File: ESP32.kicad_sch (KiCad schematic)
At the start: 5 parts, among them U1 ESP32-S3-MINI-1-N8

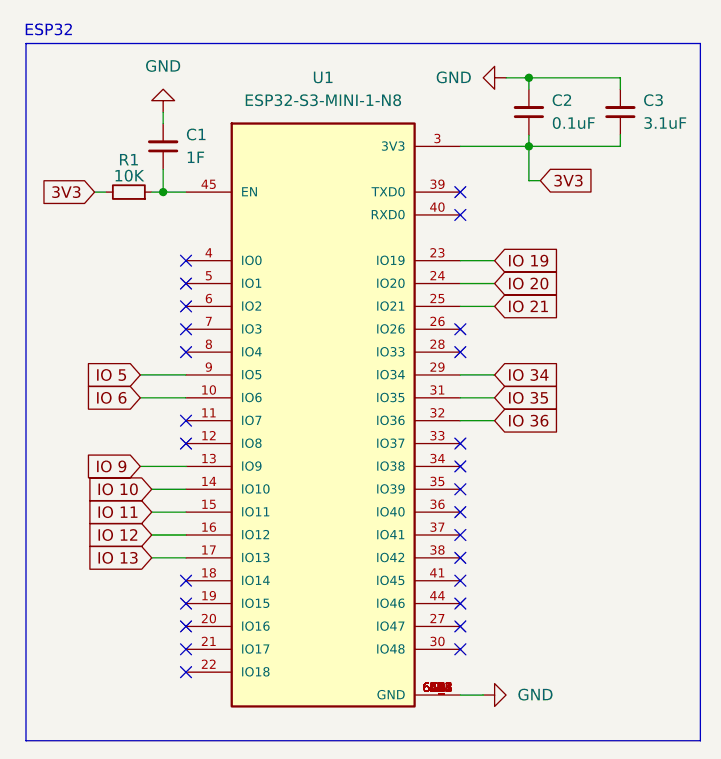
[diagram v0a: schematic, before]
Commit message: Create PCB
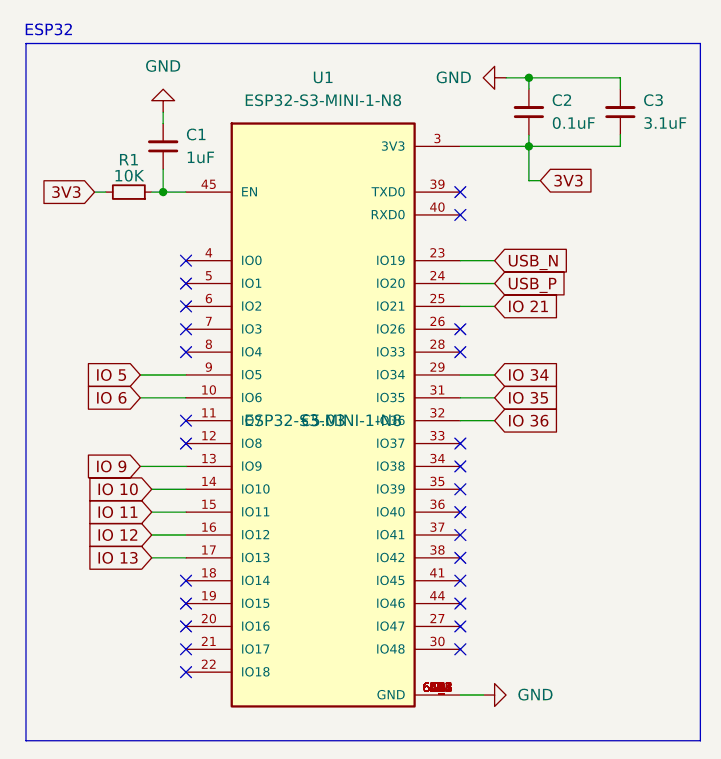
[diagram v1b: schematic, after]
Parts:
- C1: value 1F -> 1uF; DigiKey_Part_Number (none) -> 311-1445-1-ND; Manufacturer_Part_Number (none) -> CC0603KRX5R8BB105; Price (none) -> €0.95
- C2: DigiKey_Part_Number (none) -> 311-1341-1-ND; Manufacturer_Part_Number (none) -> CC0603KRX7R8BB104; Price (none) -> €0.48
- C3: footprint Capacitor_SMD:C_0603_1608Metric -> Capacitor_SMD:C_0805_2012Metric; DigiKey_Part_Number (none) -> 311-1190-1-ND; Manufacturer_Part_Number (none) -> CC0805ZKY5V6BB335; Price (none) -> €0.17
- R1: footprint Resistor_SMD:R_0603_1608Metric -> Resistor_SMD:R_0402_1005Metric; DigiKey_Part_Number (none) -> 311-10KJRCT-ND; Manufacturer_Part_Number (none) -> RC0402JR-0710KL; Price (none) -> €0.30
- U1: Check_prices https://www.snapeda.com/parts/ESP32-S3-MINI-1-N8/Espressif+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 -> (none); Description_1 Bluetooth, WiFi 802.11b/g/n, Bluetooth v5.0 Transceiver Mod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 -> (none); DigiKey_Part_Number 1965-ESP32-S3-MINI-1-N8TR-ND -> 1965-ESP32-S3-MINI-1-N8CT-ND; MANUFACTURER Espressif -> (none); MAXIMUM_PACKAGE_HEIGHT 2.55mm -> (none); MF Espressif Systems -> (none); MP ESP32-S3-MINI-1-N8 -> (none); Manufacturer_Part_Number (none) -> ESP32-S3-MINI-1-N8; PARTREV v0.6 -> (none); Package None -> (none); Price (none) -> €5.03; STANDARD Manufacturer Recommendations -> (none); SnapEDA_Link https://www.snapeda.com/parts/ESP32-S3-MINI-1-N8/Espressif+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 -> (none)
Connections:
- net IO 19 renamed USB_N
- net IO 20 renamed USB_P
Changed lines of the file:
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@@
 		)
 	)
-	(global_label "IO 19"
+	(global_label "USB_N"
 		(shape input)
 		(at 66.04 40.64 0)
@@
 		)
 		(property "Intersheetrefs" "${INTERSHEET_REFS}"
-			(at 74.3471 40.64 0)
+			(at 75.1333 40.64 0)
 			(effects
 				(font
@@
 		)
 	)
-	(global_label "IO 20"
+	(global_label "USB_P"
 		(shape input)
 		(at 66.04 43.18 0)
@@
 		)
 		(property "Intersheetrefs" "${INTERSHEET_REFS}"
-			(at 74.3471 43.18 0)
+			(at 75.0728 43.18 0)
 			(effects
 				(font
@@
 		(dnp no)
 		(fields_autoplaced yes)
-		(property "Reference" "#PWR042"
+		(property "Reference" "#PWR01"
 			(at 29.21 17.78 0)
 			(effects
@@
 			(project "RFID_Device"
 				(path "/f4733a35-9ae9-40ca-bc69-86dc96557334/b59a840b-0db4-4dd4-af14-dad68e1751ca"
-					(reference "#PWR042")
+					(reference "#PWR01")
 					(unit 1)
 				)
@@
 			)
 		)
-		(property "Value" "1F"
+		(property "Value" "1uF"
 			(at 31.75 29.2035 0)
 			(effects
@@
 		)
 		(property "Description" "Unpolarized capacitor, small symbol"
+			(at 29.21 27.94 0)
+			(effects
+				(font
+					(size 1.27 1.27)
+				)
+				(hide yes)
+			)
+		)
+		(property "DigiKey_Part_Number" "311-1445-1-ND"
+			(at 29.21 27.94 0)
+			(effects
+				(font
+					(size 1.27 1.27)
+				)
+				(hide yes)
+			)
+		)
+		(property "Manufacturer_Part_Number" "CC0603KRX5R8BB105"
+			(at 29.21 27.94 0)
+			(effects
+				(font
+					(size 1.27 1.27)
+				)
+				(hide yes)
+			)
+		)
+		(property "Price" "€0.95"
 			(at 29.21 27.94 0)
 			(effects
@@
 			)
 		)
-		(property "Footprint" "Capacitor_SMD:C_0603_1608Metric"
+		(property "Footprint" "Capacitor_SMD:C_0805_2012Metric"
 			(at 80.01 24.13 0)
 			(effects
@@
 		)
 		(property "Description" "Unpolarized capacitor, small symbol"
+			(at 80.01 24.13 0)
+			(effects
+				(font
+					(size 1.27 1.27)
+				)
+				(hide yes)
+			)
+		)
+		(property "Price" "€0.17"
+			(at 80.01 24.13 0)
+			(effects
+				(font
+					(size 1.27 1.27)
+				)
+				(hide yes)
+			)
+		)
+		(property "DigiKey_Part_Number" "311-1190-1-ND"
+			(at 80.01 24.13 0)
+			(effects
+				(font
+					(size 1.27 1.27)
+				)
+				(hide yes)
+			)
+		)
+		(property "Manufacturer_Part_Number" "CC0805ZKY5V6BB335"
 			(at 80.01 24.13 0)
 			(effects
@@
 			)
 		)
-		(property "DigiKey_Part_Number" "1965-ESP32-S3-MINI-1-N8TR-ND"
+		(property "DigiKey_Part_Number" "1965-ESP32-S3-MINI-1-N8CT-ND"
 			(at 46.99 58.42 0)
 			(effects
@@
 			)
 		)
-		(property "SnapEDA_Link" "https://www.snapeda.com/parts/ESP32-S3-MINI-1-N8/Espressif+Systems/view-part/?ref=snap"
+		(property "Price" "€5.03"
 			(at 46.99 58.42 0)
 			(effects
@@
 					(size 1.27 1.27)
 				)
-				(justify bottom)
-				(hide yes)
-			)
-		)
-		(property "MAXIMUM_PACKAGE_HEIGHT" "2.55mm"
+			)
+		)
+		(property "Manufacturer_Part_Number" "ESP32-S3-MINI-1-N8"
 			(at 46.99 58.42 0)
 			(effects
@@
 					(size 1.27 1.27)
 				)
-				(justify bottom)
-				(hide yes)
-			)
-		)
-		(property "Package" "None"
-			(at 46.99 58.42 0)
-			(effects
-				(font
-					(size 1.27 1.27)
-				)
-				(justify bottom)
-				(hide yes)
-			)
-		)
-		(property "Check_prices" "https://www.snapeda.com/parts/ESP32-S3-MINI-1-N8/Espressif+Systems/view-part/?ref=eda"
-			(at 46.99 58.42 0)
-			(effects
-				(font
-					(size 1.27 1.27)
-				)
-				(justify bottom)
-				(hide yes)
-			)
-		)
-		(property "STANDARD" "Manufacturer Recommendations"
-			(at 46.99 58.42 0)
-			(effects
-				(font
-					(size 1.27 1.27)
-				)
-				(justify bottom)
-				(hide yes)
-			)
-		)
-		(property "PARTREV" "v0.6"
-			(at 46.99 58.42 0)
-			(effects
-				(font
-					(size 1.27 1.27)
-				)
-				(justify bottom)
-				(hide yes)
-			)
-		)
-		(property "MF" "Espressif Systems"
-			(at 46.99 58.42 0)
-			(effects
-				(font
-					(size 1.27 1.27)
-				)
-				(justify bottom)
-				(hide yes)
-			)
-		)
-		(property "MP" "ESP32-S3-MINI-1-N8"
-			(at 46.99 58.42 0)
-			(effects
-				(font
-					(size 1.27 1.27)
-				)
-				(justify bottom)
-				(hide yes)
-			)
-		)
-		(property "Description_1" "\n                        \n                            Bluetooth, WiFi 802.11b/g/n, Bluetooth v5.0 Transceiver Module 2.4GHz PCB Trace Surface Mount\n                        \n"
-			(at 46.99 58.42 0)
-			(effects
-				(font
-					(size 1.27 1.27)
-				)
-				(justify bottom)
-				(hide yes)
-			)
-		)
-		(property "MANUFACTURER" "Espressif"
-			(at 46.99 58.42 0)
-			(effects
-				(font
-					(size 1.27 1.27)
-				)
-				(justify bottom)
-				(hide yes)
 			)
 		)
@@
 			)
 		)
-		(property "Footprint" "Resistor_SMD:R_0603_1608Metric"
+		(property "Footprint" "Resistor_SMD:R_0402_1005Metric"
 			(at 25.4 33.02 0)
 			(effects
@@
 		)
 		(property "Description" "Resistor, small symbol"
+			(at 25.4 33.02 0)
+			(effects
+				(font
+					(size 1.27 1.27)
+				)
+				(hide yes)
+			)
+		)
+		(property "Price" "€0.30"
+			(at 25.4 33.02 0)
+			(effects
+				(font
+					(size 1.27 1.27)
+				)
+				(hide yes)
+			)
+		)
+		(property "DigiKey_Part_Number" "311-10KJRCT-ND"
+			(at 25.4 33.02 0)
+			(effects
+				(font
+					(size 1.27 1.27)
+				)
+				(hide yes)
+			)
+		)
+		(property "Manufacturer_Part_Number" "RC0402JR-0710KL"
 			(at 25.4 33.02 0)
 			(effects
@@
 			(at 69.85 24.13 0)
 			(effects
+				(font
+					(size 1.27 1.27)
+				)
+				(hide yes)
+			)
+		)
+		(property "DigiKey_Part_Number" "311-1341-1-ND"
+			(at 69.85 24.13 0)
+			(effects
+				(font
+					(size 1.27 1.27)
+				)
+				(hide yes)
+			)
+		)
+		(property "Price" "€0.48"
+			(at 69.85 24.13 0)
+			(effects
+				(font
+					(size 1.27 1.27)
+				)
+				(hide yes)
+			)
+		)
+		(property "Manufacturer_Part_Number" "CC0603KRX7R8BB104"
+			(at 69.85 24.13 0)
+			(effects
